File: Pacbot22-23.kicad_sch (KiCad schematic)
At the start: 0 parts

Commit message: My schtuff
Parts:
- added C1, C2: 15pF, symbol Device:C_Small
- added C10: 1uF, symbol Device:C_Small
- added R10, R20: 10k, symbol Device:R_Small
- added SW1: SW_Push, symbol Switch:SW_Push
- added U1: ATmega32U4-A, Package_QFP:TQFP-44_10x10mm_P0.8mm, symbol MCU_Microchip_ATmega:ATmega32U4-A
- added Y1: 16Mhz, symbol Device:Crystal_Small
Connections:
- new net +5V: R10.1, U1.14 (VCC), U1.2 (UVCC), U1.24 (AVCC), U1.34 (VCC), U1.42 (AREF), U1.44 (AVCC), U1.7 (VBUS)
- new net BNO_INT: U1.39 (PF4)
- new net D+: U1.4 (D+)
- new net D-: U1.3 (D-)
- new net ENC11: U1.28 (PB4)
- new net ENC12: U1.29 (PB5)
- new net ENC21: U1.8 (PB0)
- new net ENC22: U1.9 (PB1)
- new net GND: C1.1, C10.2, C2.1, R20.2, SW1.1, U1.15 (GND), U1.23 (GND), U1.35 (GND), U1.43 (GND), U1.5 (UGND)
- new net M11: U1.26 (PD6)
- new net M12: U1.27 (PD7)
- new net M21: U1.10 (PB2)
- new net M22: U1.11 (PB3)
- new net PB6: U1.30 (PB6)
- new net PB7: U1.12 (PB7)
- new net PC6: U1.31 (PC6)
- new net PC7: U1.32 (PC7)
- new net PD4: U1.25 (PD4)
- new net PD5: U1.22 (PD5)
- new net PE2: R20.1, U1.33 (~{HWB}/PE2)
- new net PE6: U1.1 (PE6)
- new net PF5: U1.38 (PF5)
- new net PF6: U1.37 (PF6)
- new net PF7: U1.36 (PF7)
- new net RX: U1.20 (PD2)
- new net SCL: U1.18 (PD0)
- new net SDA: U1.19 (PD1)
- new net SR_C: U1.41 (PF0)
- new net SR_D: U1.40 (PF1)
- new net TX: U1.21 (PD3)
- new net UCAP: C10.1, U1.6 (UCAP)
- new net XTAL1: C1.2, U1.17 (XTAL1), Y1.1
- new net XTAL2: C2.2, U1.16 (XTAL2), Y1.2
- new net ~{RESET}: R10.2, SW1.2, U1.13 (~{RESET})
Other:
- added sheet TestPoints (TestPoints.kicad_sch)
- note added: "ATMEGA32u4"
- note added: "BNO055 IMU"
- note added: "Decoupling Capacitors"
- note added: "Distance Sensors"
- note added: "H-Bridges"
- note added: "Motor Connectors"
- note added: "Power Term"
- note added: "Shift Reg"
- note added: "USB Connector"

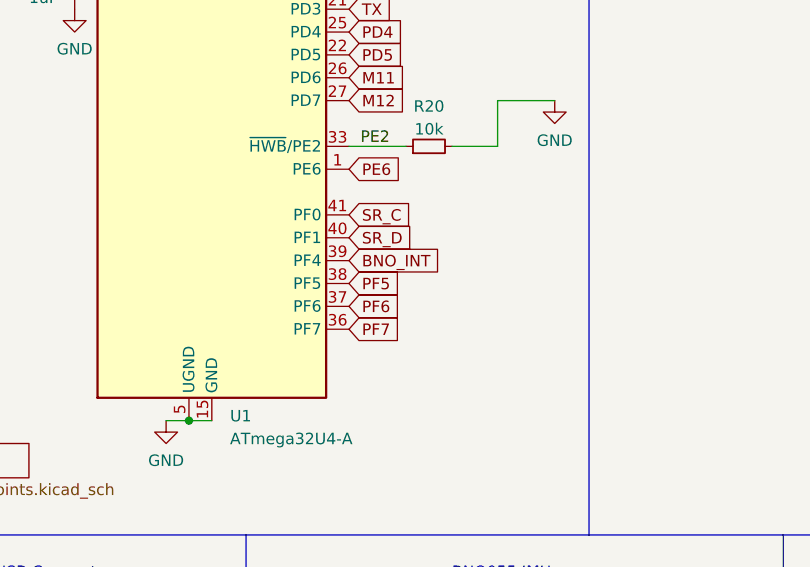
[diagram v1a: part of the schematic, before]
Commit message: Updated libs
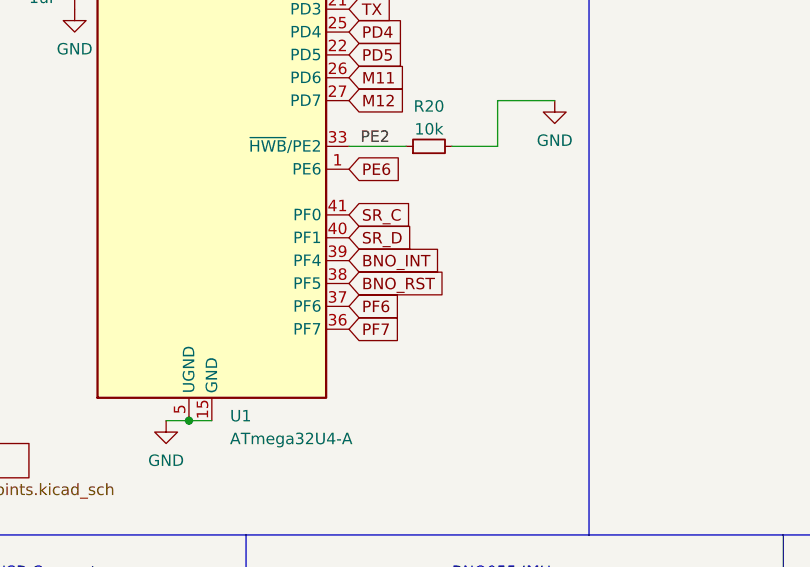
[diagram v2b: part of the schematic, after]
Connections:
- net PF5 renamed BNO_RST
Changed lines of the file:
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@@
     )
   )
-  (global_label "PF5" (shape input) (at 62.23 114.3 0) (fields_autoplaced)
+  (global_label "BNO_RST" (shape input) (at 62.23 114.3 0) (fields_autoplaced)
     (effects (font (size 1.27 1.27)) (justify left))
-    (property "Intersheet References" "${INTERSHEET_REFS}" (id 0) (at 68.2112 114.2206 0)
+    (property "Intersheet References" "${INTERSHEET_REFS}" (id 0) (at 72.9888 114.2206 0)
       (effects (font (size 1.27 1.27)) (justify left) hide)
     )
